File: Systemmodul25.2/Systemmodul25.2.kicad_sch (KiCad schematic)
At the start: 34 parts, among them J1 DIN41612_02x16_AB, J2 DIN41612_02x16_AB, J3 AVR-ISP-6, Q1 12.00J1, U1 W27E040, U2 W27E040, U3 M48T18-100PC1, U4 ATmega8515-16A, U5 MAX690xPA

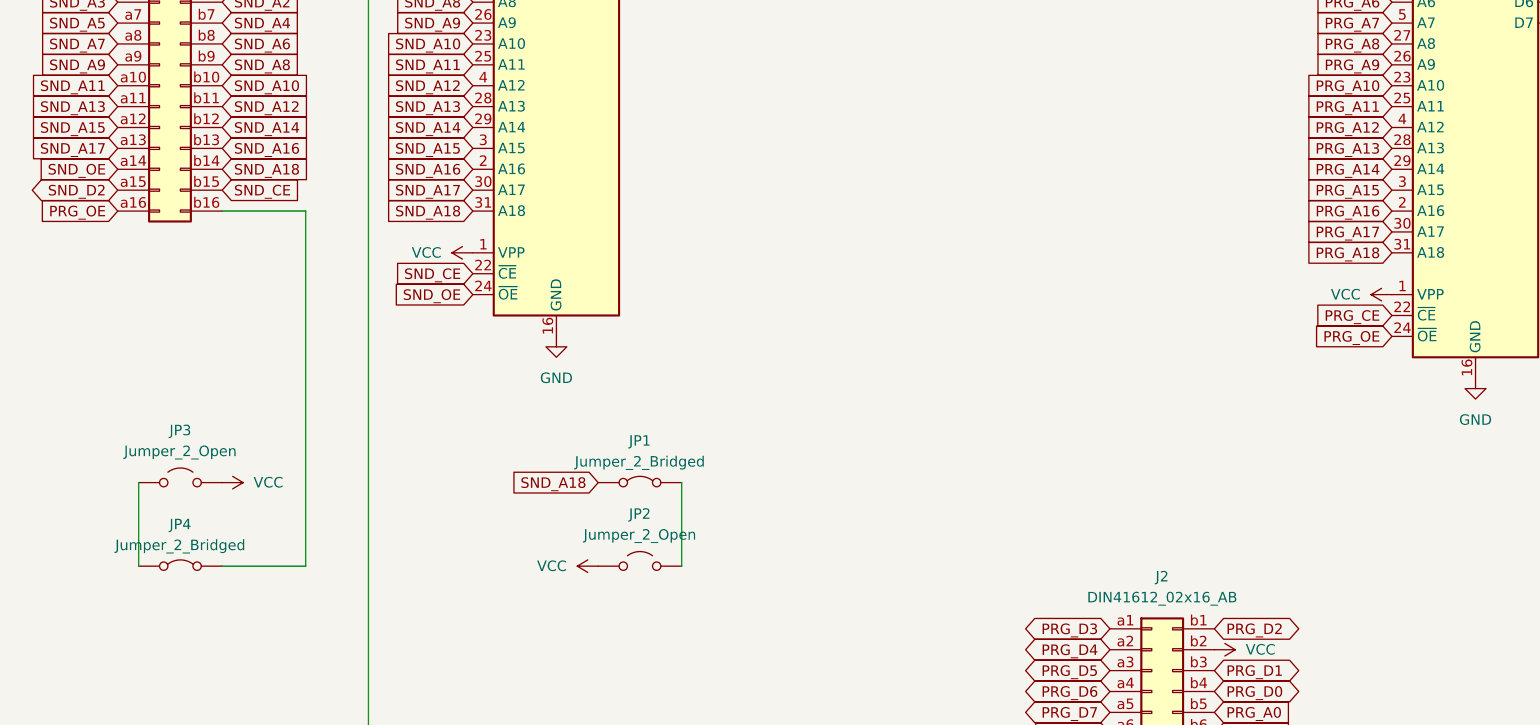
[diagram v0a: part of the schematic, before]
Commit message: systemmodul fertig
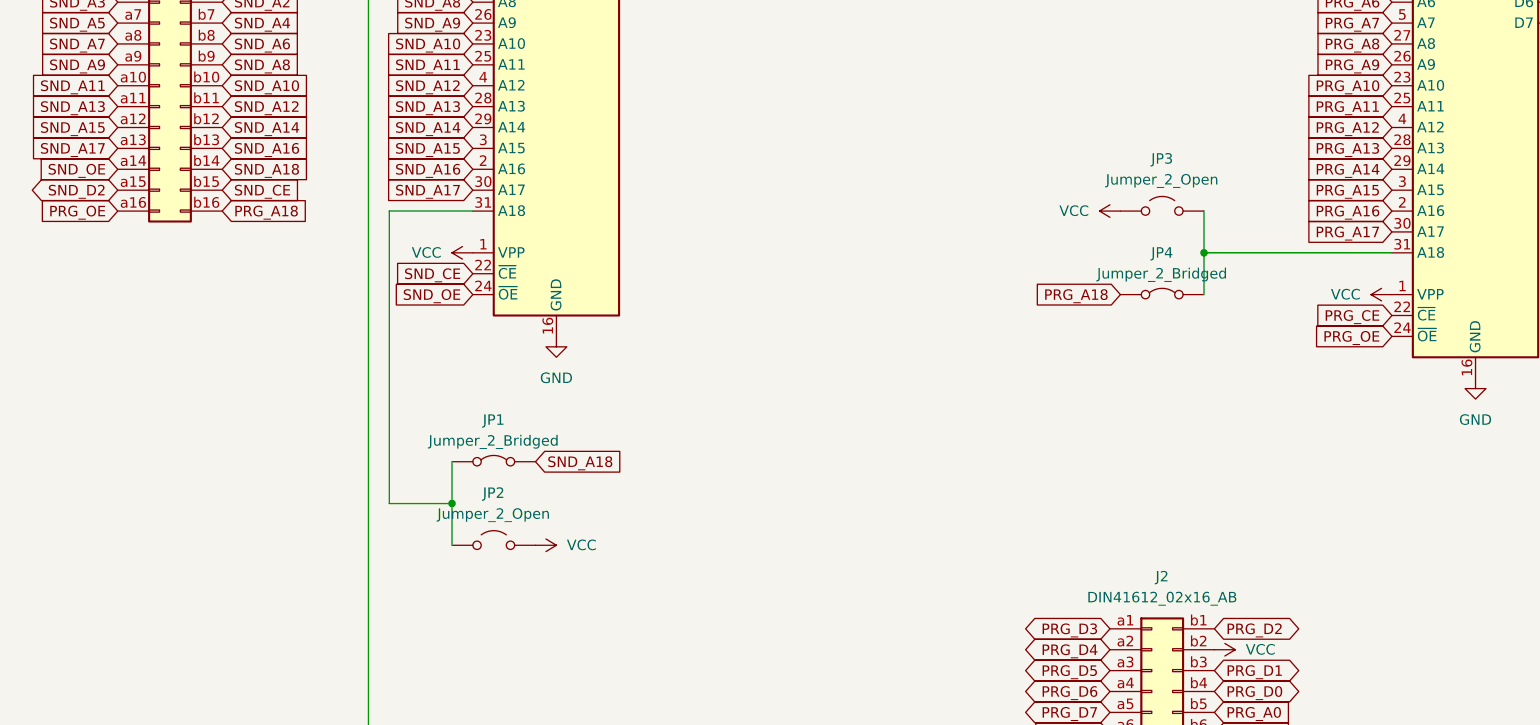
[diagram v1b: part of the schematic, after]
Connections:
- net PRG_A18: now also J1.b16 (Pin_b16), JP4.2 (B); no longer U2.31 (A18)
- net SND_A18: no longer U1.31 (A18)
- net at JP1.1 (A), JP2.1 (A): now also U1.31 (A18)
- net at JP3.1 (A), JP4.1 (A): now also U2.31 (A18)
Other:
- moved on the sheet: JP1, JP2, JP3, JP4

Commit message: systemmodul reset
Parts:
- removed FID5: Fiducial, symbol Mechanical:Fiducial
- D1: value D -> BAT85
- FID1, FID2: footprint Fiducial:Fiducial_Cross_0.5mm_Mask2mm -> Fiducial:Fiducial_Cross_1.5mm_Mask2mm
- FID3: footprint (none) -> Fiducial:Fiducial_0.75mm_Mask1.5mm
- JP1: value Jumper_2_Bridged -> Sound_4MBit
- JP2: value Jumper_2_Open -> Sound_2MBit
- JP3: value Jumper_2_Open -> Program_2MBit
- JP4: value Jumper_2_Bridged -> Program_4MBit
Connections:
- net GND: now also U5.4 (PFI)
- net RESET: now reaches J3.5 (~{RST}), U4.4 (~{RESET})
- net RESET: now also R4.2, U5.7 (~{RESET})
- no-connect marks 3 -> 13
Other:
- moved on the sheet: C1, C2, C3, C4, C5, C6, C8, C9, D1, FID1, FID2, FID3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
